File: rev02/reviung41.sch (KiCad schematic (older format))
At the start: 85 parts, among them SW10 SW_PUSH, SW11 SW_PUSH, SW12 SW_PUSH, SW14 SW_PUSH, SW15 SW_PUSH, SW16 SW_PUSH, SW17 SW_PUSH, SW18 SW_PUSH, SW19 SW_PUSH, SW2 SW_PUSH, SW20 SW_PUSH, SW21 SW_PUSH, SW22 SW_PUSH, SW23 SW_PUSH, SW25 SW_PUSH, SW26 SW_PUSH, SW27 SW_PUSH, SW28 SW_PUSH, SW29 SW_PUSH, SW3 SW_PUSH, SW31 SW_PUSH, SW32 SW_PUSH, SW33 SW_PUSH, SW34 SW_PUSH, SW35 SW_PUSH, SW37 SW_PUSH, SW38 SW_PUSH, SW39 SW_PUSH, SW4 SW_PUSH, SW40 SW_PUSH, SW41 SW_PUSH, SW42 SW_PUSH, SW5 SW_PUSH, SW6 SW_PUSH, SW8 SW_PUSH, SW9 SW_PUSH, U1 ProMicro

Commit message: Some major changes, replaced diodes with SOD123, fixed some routing, updated footprints to use different libraries
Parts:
- D10, D11, D12, D14, D15, D16, D17, D18, D19, D2, D20, D21, D22, D23, D25, D26, D27, D28, D29, D3, D31, D32, D33, D34, D35, D37, D38, D39, D4, D40, D41, D42, D5, D6, D8, D9: footprint _reviung-kbd:D3_SMD_1side -> Diode_SMD:D_SOD-123
- L1, L10, L11, L2, L3, L4, L5, L6, L7, L8, L9: footprint _reviung-kbd:LED_WS2812B_PLCC4_5.0x5.0mm_P3.2mm -> LED_SMD:LED_WS2812B_PLCC4_5.0x5.0mm_P3.2mm

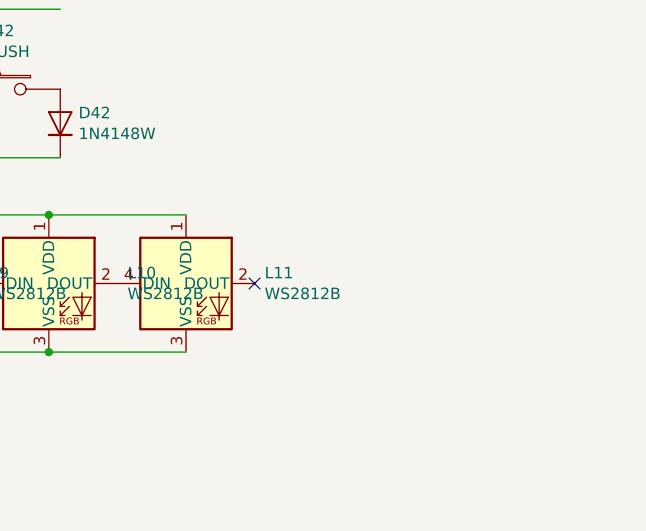
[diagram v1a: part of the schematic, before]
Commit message: euclid36 rev, sent to production...
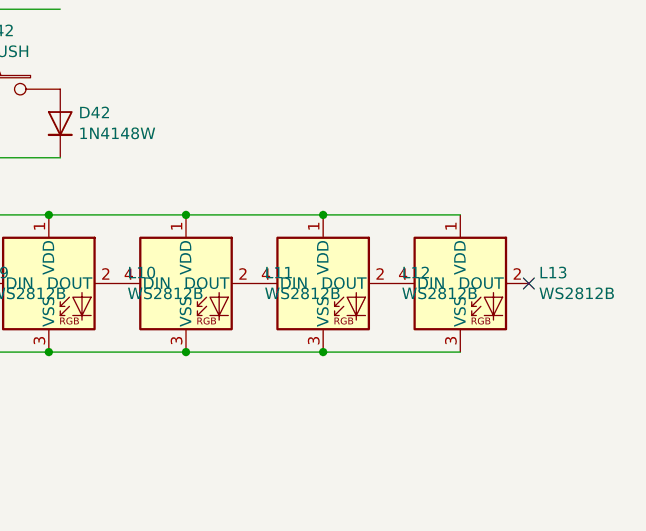
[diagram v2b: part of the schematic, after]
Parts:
- added L12, L13: WS2812B, LED_SMD:LED_WS2812B_PLCC4_5.0x5.0mm_P3.2mm, symbol reviung41-rescue:WS2812B-LED
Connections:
- net GND: now also L12.3 (VSS), L13.3 (VSS)
- net VCC: now also L12.1 (VDD), L13.1 (VDD)
- net at L11.2 (DOUT): now also L12.4 (DIN)
- new net: L12.2 (DOUT), L13.4 (DIN)
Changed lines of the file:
@@
 	1    0    0    -1
 $EndComp
-NoConn ~ 9750 6100
 Wire Wire Line
 	3250 5800 3450 5800
@@
 	8900 5550 7900 5550
 Connection ~ 7900 5550
+$Comp
+L reviung41-rescue:WS2812B-LED L12
+U 1 1 6059142A
+P 10050 6100
+F 0 "L12" H 10394 6146 50  0000 L CNN
+F 1 "WS2812B" H 10394 6055 50  0000 L CNN
+F 2 "LED_SMD:LED_WS2812B_PLCC4_5.0x5.0mm_P3.2mm" H 10100 5800 50  0001 L TNN
+F 3 "https://cdn-shop.adafruit.com/datasheets/WS2812B.pdf" H 10150 5725 50  0001 L TNN
+	1    10050 6100
+	1    0    0    -1
+$EndComp
+Wire Wire Line
+	9450 5800 10050 5800
+Wire Wire Line
+	9450 6400 10050 6400
+$Comp
+L reviung41-rescue:WS2812B-LED L13
+U 1 1 6059DED0
+P 10650 6100
+F 0 "L13" H 10994 6146 50  0000 L CNN
+F 1 "WS2812B" H 10994 6055 50  0000 L CNN
+F 2 "LED_SMD:LED_WS2812B_PLCC4_5.0x5.0mm_P3.2mm" H 10700 5800 50  0001 L TNN
+F 3 "https://cdn-shop.adafruit.com/datasheets/WS2812B.pdf" H 10750 5725 50  0001 L TNN
+	1    10650 6100
+	1    0    0    -1
+$EndComp
+Wire Wire Line
+	10050 5800 10650 5800
+Wire Wire Line
+	10050 6400 10650 6400
+Connection ~ 9450 5800
+Connection ~ 9450 6400
+Connection ~ 10050 5800
+Connection ~ 10050 6400
+NoConn ~ 10950 6100
 $EndSCHEMATC
